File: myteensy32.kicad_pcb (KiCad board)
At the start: 2 copper layers, 35.6 x 17.8 mm, 31 parts, among them J1 Conn_01x14_Male, J2 Conn_01x14_Male, J3 USB_C_Receptacle_USB2.0, SW1 RESET, SW2 PROG, U1 MKL04Z32VLC4, U2 MK20DX256VLH7, U3 MCP2562-E-SN, U4 NJM2884U1, Y2 16MHz

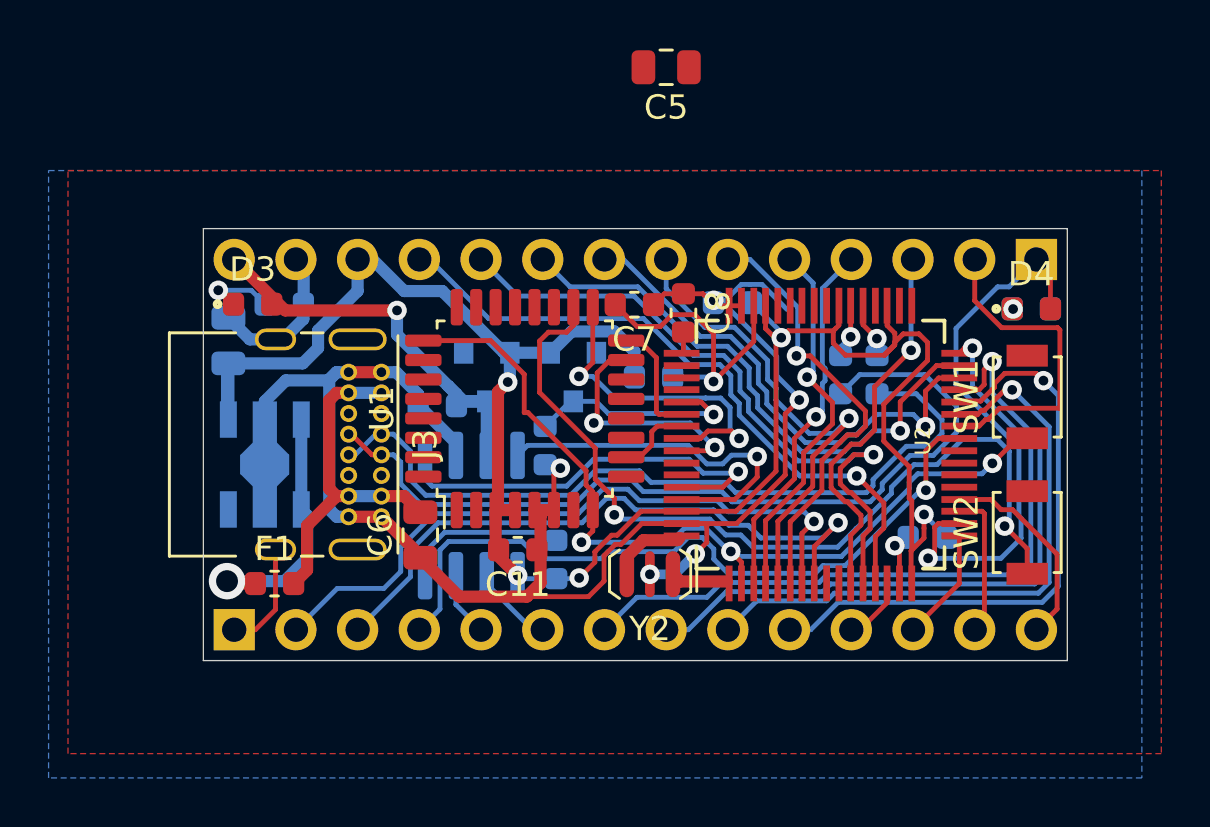
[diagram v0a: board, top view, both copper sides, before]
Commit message: いったんコミット
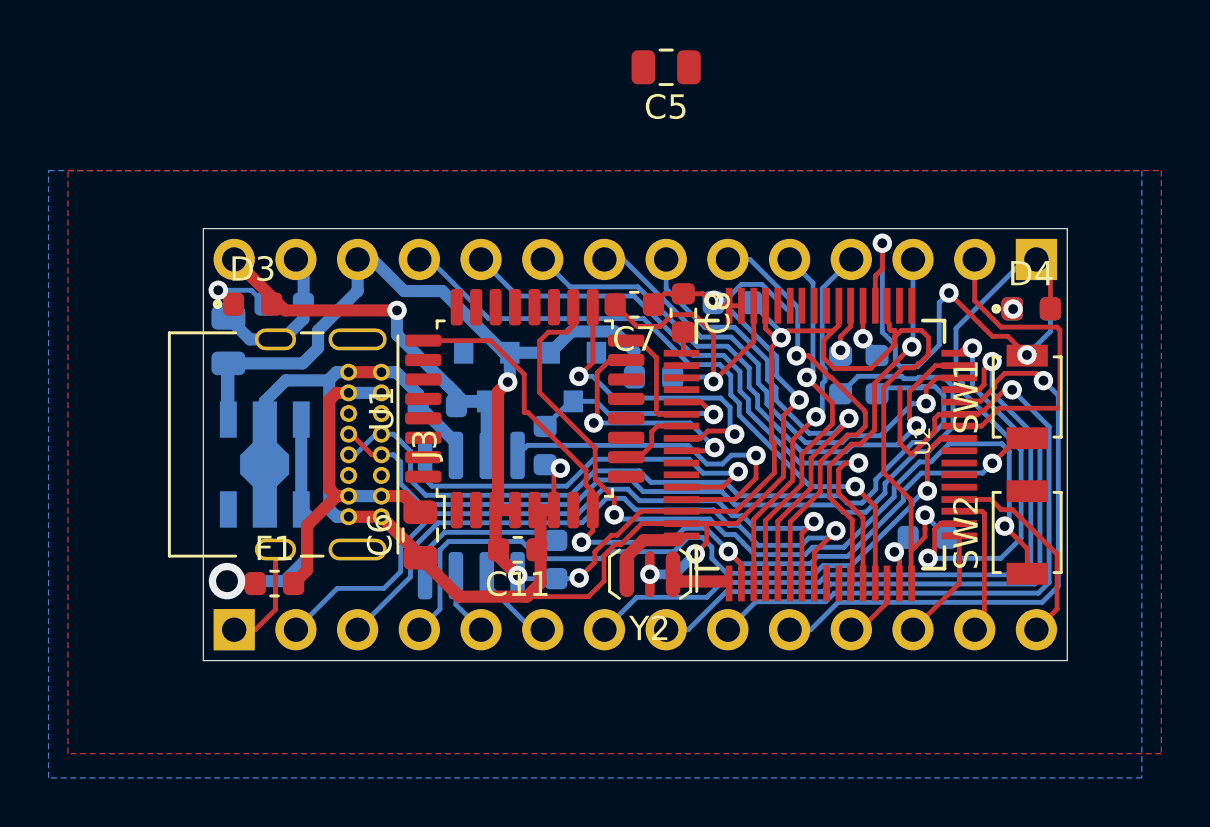
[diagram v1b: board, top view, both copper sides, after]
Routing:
- net GND: track 91.0 -> 109.8 mm, vias 6 -> 9
- net Net-(J2-Pad9): track 25.2 -> 31.1 mm
- net Net-(J1-Pad10): track 27.5 -> 25.8 mm
- net +3V3: track 85.7 -> 87.3 mm
- net /USB+: track 32.2 -> 33.3 mm
- net Net-(J1-Pad8): track 20.9 -> 20.0 mm
- net Net-(J1-Pad11): track 27.5 -> 26.9 mm
- net Net-(J1-Pad9): track 23.3 -> 23.9 mm
- net /PTA2: track 13.9 -> 13.4 mm
